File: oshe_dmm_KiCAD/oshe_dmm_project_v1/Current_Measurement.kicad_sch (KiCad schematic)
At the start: 2 parts

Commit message: Update Current_Measurement.kicad_sch
deleted
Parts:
- removed C1: C, symbol Device:C
- removed R1: R_US, symbol Device:R_US
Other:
- note removed: "Random test circuit to test file sharing, delete this!"

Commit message: Added Current Measurement
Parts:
- added C1: 0.1u, Capacitor_SMD:C_0201_0603Metric_Pad0.64x0.40mm_HandSolder, symbol Device:C
- added R1: .064R, Resistor_SMD:R_2512_6332Metric_Pad1.40x3.35mm_HandSolder, symbol Device:R
- added R2: 1k, Resistor_SMD:R_0603_1608Metric_Pad0.98x0.95mm_HandSolder, symbol Device:R
- added R3: 1K, Resistor_SMD:R_0603_1608Metric_Pad0.98x0.95mm_HandSolder, symbol Device:R
- added U1: INA219BxD, Package_SO:SOIC-8_3.9x4.9mm_P1.27mm, symbol Sensor_Energy:INA219BxD
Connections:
- new net: R2.2, U1.1 (A1)
- new net: R3.2, U1.2 (A0)
- new net Current Negative: R1.2, U1.7 (IN-)
- new net Current Positive: R1.1, U1.8 (IN+)
- new net GND: C1.1, R2.1, R3.1, U1.6 (GND)
- new net SCL: U1.4 (SCL)
- new net SDA: U1.3 (SDA)
- new net VCC: C1.2, U1.5 (VS)

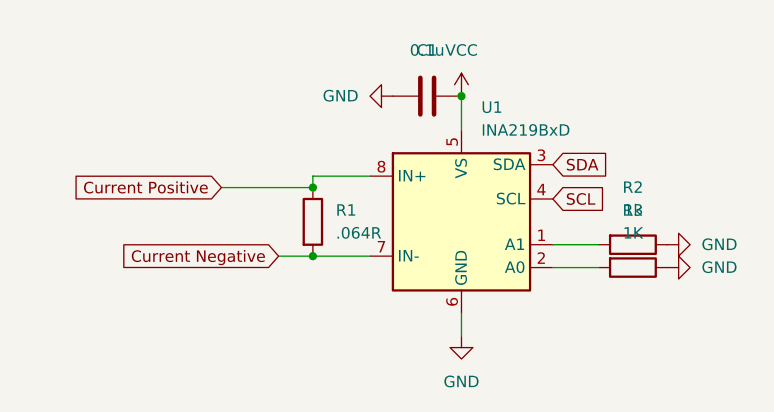
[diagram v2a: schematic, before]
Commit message: Made changes to PCB and Schematic
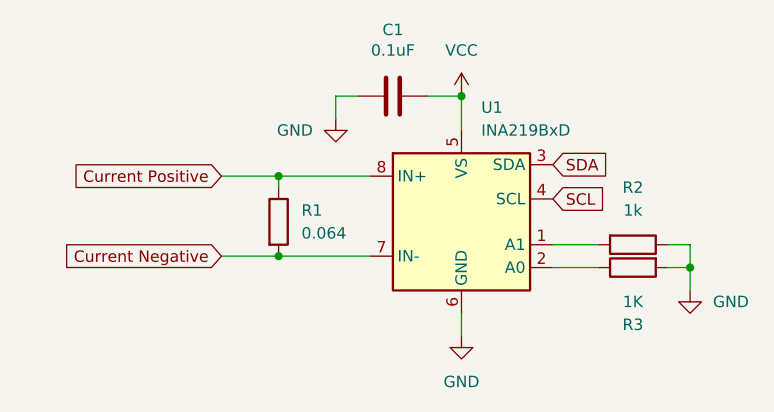
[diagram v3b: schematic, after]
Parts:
- C1: value 0.1u -> 0.1uF
- R1: value .064R -> 0.064
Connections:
- net GND: now also R3.2; no longer R3.1
- net at U1.2 (A0): now also R3.1; no longer R3.2
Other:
- moved on the sheet: C1, R1, R3
